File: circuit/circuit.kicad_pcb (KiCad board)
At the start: 4 copper layers, 175.5 x 119.5 mm, 206 parts, among them J201 Barrel_Jack, J301 FX_R_2, J302 FX_R_4, J303 FX_R_6, J304 FX_R_8, J305 FX_R_1, J306 FX_R_3, J307 FX_R_5, J308 FX_R_7, J309 FX_S_1, J310 FX_S_2, J311 FX_S_3, J312 FX_S_4, J313 FX_S_5, J314 FX_S_6, J315 FX_S_7, J316 FX_S_8, J317 Guitar_In, J318 Amp_Out, SW101 Pedal_1, SW102 Pedal_2, SW103 Pedal_3, SW104 Pedal_4, SW105 Pedal_5, SW106 Pedal_6, SW107 Pedal_7, SW108 Pedal_8, SW109 Program, SW110 Preset, U101 ESP32-S3-DevKitC, U201 TMA-1215D, U202 LM7805_TO220, U203 LM7905_TO220, U204 LM1117T-3.3, U301 TL072, U302 TL072, U303 TL072, U304 TL072, U305 TL072, U306 TL072, U307 TL072, U308 TL072, U309 TL072, U401 ADG419BN, U402 CD4051B, U501 CD4051B, U502 CD4051B, U503 CD4051B, U504 CD4051B, U601 CD4051B, U602 CD4051B, U603 CD4051B, U604 CD4051B, U701 74HC595, U702 74HC595, U703 74HC595, U704 74HC595, U801 74HC595, U802 74HC595, U901 74HC595, U902 74HC595

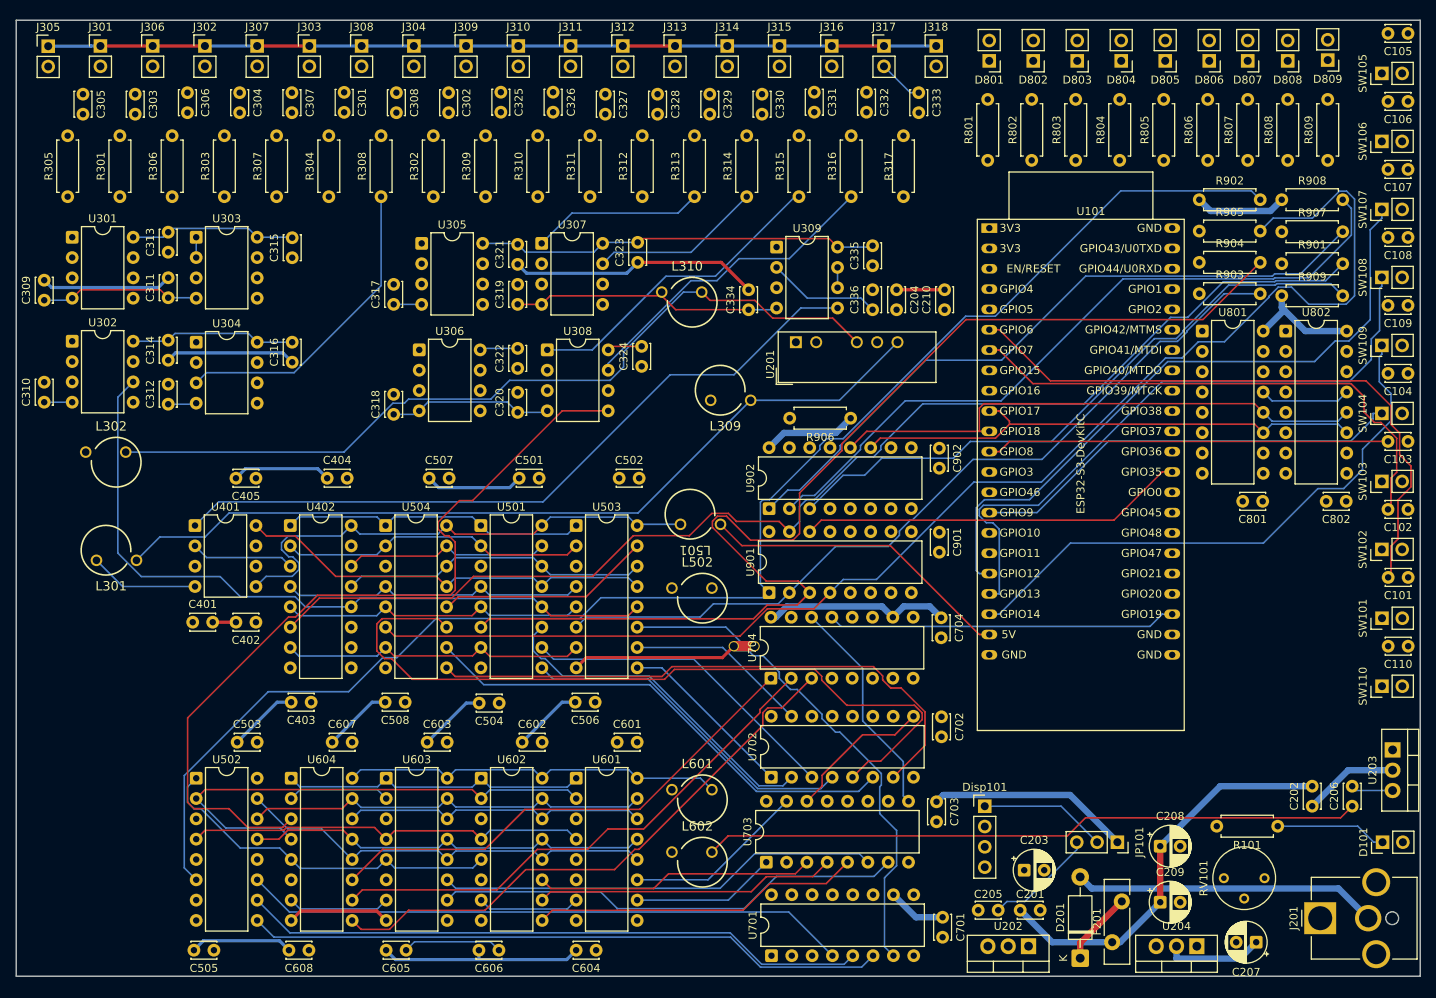
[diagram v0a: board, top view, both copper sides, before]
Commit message: Circuit tweaks and PCB
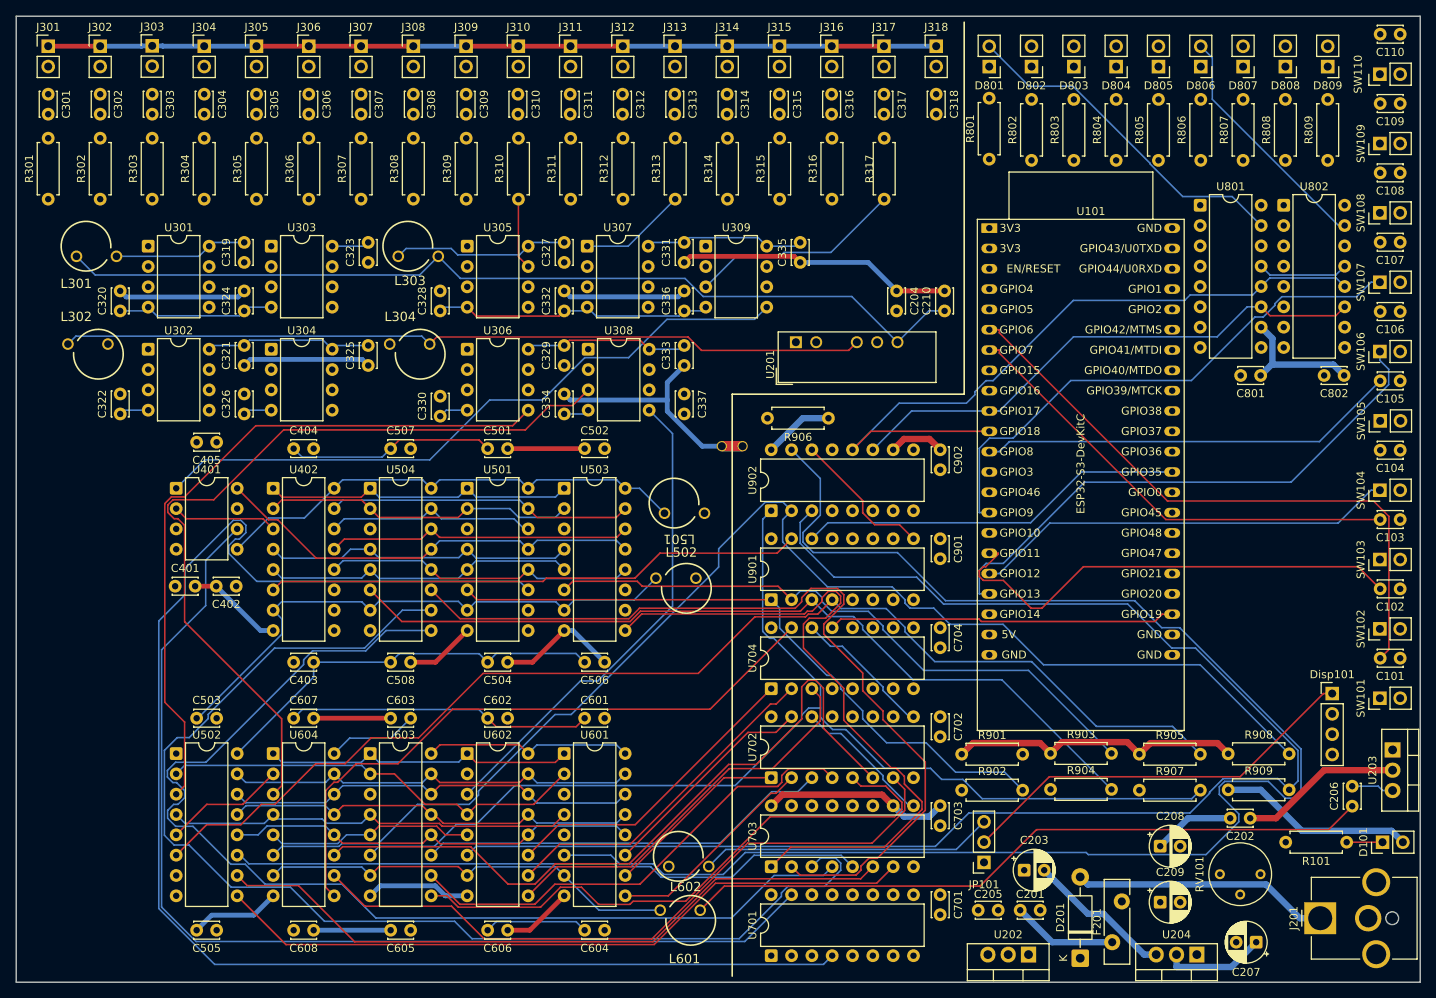
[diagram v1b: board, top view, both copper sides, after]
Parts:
- removed L309, L310: 600R@100Mhz, WE-UKW:WE-UKW_74275010
- added C337: 1uF, Capacitor_THT:C_Disc_D3.0mm_W2.0mm_P2.50mm, F.Cu at (122.0, 84.0)
- added L303: 600R@100Mhz, WE-UKW:WE-UKW_74275010, F.Cu at (87.5, 65.5)
- added L304: 600R@100Mhz, WE-UKW:WE-UKW_74275010, F.Cu at (89.0, 79.0)
- C309, C310, C311, C312, C313, C314, C315, C316, C317, C318: value 0.1uF -> 1uF
- C325, C326, C327, C328, C329, C330, C331, C332, C333, C336: value 1uF -> 0.1uF
- D201: value 1N4007 -> 1N5822
- J301: value FX_R_2 -> FX_R_1
- J302: value FX_R_4 -> FX_R_2
- J303: value FX_R_6 -> FX_R_3
- J304: value FX_R_8 -> FX_R_4
- J305: value FX_R_1 -> FX_R_5
- J306: value FX_R_3 -> FX_R_6
- J307: value FX_R_5 -> FX_R_7
- J308: value FX_R_7 -> FX_R_8
- SW102: value Pedal_2 -> Pedal_6
- SW103: value Pedal_3 -> Pedal_2
- SW104: value Pedal_4 -> Pedal_7
- SW105: value Pedal_5 -> Pedal_3
- SW106: value Pedal_6 -> Pedal_8
- SW107: value Pedal_7 -> Pedal_4
- SW108: value Pedal_8 -> Program
- SW109: value Program -> Pedal_5
- moved R902 79.6 mm to (156.7, 133.5)
- moved C318 78.7 mm to (153.5, 46.5), turned to -90 degrees
- moved C314 77.4 mm to (127.4, 46.5), turned to -90 degrees
- moved C110 76.5 mm to (211.5, 39.0)
- moved SW110 76.5 mm to (209.0, 44.0)
- moved C316 75.3 mm to (140.4, 46.5), turned to -90 degrees
- moved R901 73.2 mm to (156.7, 129.0)
- moved R907 72.0 mm to (178.9, 133.5)
- moved C310 70.6 mm to (101.2, 46.5), turned to -90 degrees
- moved R908 69.6 mm to (190.0, 128.9)
- moved C312 68.7 mm to (114.3, 46.5), turned to -90 degrees
- moved R904 68.4 mm to (167.8, 133.4)
- moved C317 66.7 mm to (147.0, 46.5), turned to -90 degrees
- moved C313 66.3 mm to (120.8, 46.5), turned to -90 degrees
- moved R905 65.8 mm to (178.9, 129.0)
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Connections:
- C102 pad 2: Net-(U101-GPIO7/ADC1_CH6) -> Net-(U101-GPIO11/ADC2_CH0)
- C103 pad 2: Net-(U101-GPIO8/ADC1_CH7) -> Net-(U101-GPIO7/ADC1_CH6)
- C104 pad 2: Net-(U101-GPIO9/ADC1_CH8) -> Net-(U101-GPIO12/ADC2_CH1)
- C105 pad 2: Net-(U101-GPIO10/ADC1_CH9) -> Net-(U101-GPIO8/ADC1_CH7)
- C106 pad 2: Net-(U101-GPIO11/ADC2_CH0) -> Net-(U101-GPIO13/ADC2_CH2)
- C107 pad 2: Net-(U101-GPIO12/ADC2_CH1) -> Net-(U101-GPIO9/ADC1_CH8)
- C108 pad 2: Net-(U101-GPIO13/ADC2_CH2) -> Net-(U101-GPIO14/ADC2_CH3)
- C109 pad 2: Net-(U101-GPIO14/ADC2_CH3) -> Net-(U101-GPIO10/ADC1_CH9)
- C309 pad 1: _15V_F -> Net-(C309-Pad1)
- C309 pad 2: AGND -> Net-(C309-Pad2)
- C310 pad 1: _15V_F -> Net-(C310-Pad1)
- C310 pad 2: AGND -> Net-(C310-Pad2)
- C311 pad 1: _15V_F -> Net-(C311-Pad1)
- C311 pad 2: AGND -> Net-(C311-Pad2)
- C312 pad 1: _15V_F -> Net-(C312-Pad1)
- C312 pad 2: AGND -> Net-(C312-Pad2)
- C313 pad 1: AGND -> Net-(C313-Pad1)
- C313 pad 2: +15V_F -> Net-(C313-Pad2)
- C314 pad 1: AGND -> Net-(C314-Pad1)
- C314 pad 2: +15V_F -> Net-(C314-Pad2)
- C315 pad 1: AGND -> Net-(C315-Pad1)
- C315 pad 2: +15V_F -> Net-(C315-Pad2)
- C316 pad 1: AGND -> Net-(C316-Pad1)
- C316 pad 2: +15V_F -> Net-(C316-Pad2)
- C317 pad 1: Net-(U305-V-) -> Net-(C317-Pad1)
- C317 pad 2: AGND -> Net-(C317-Pad2)
- C318 pad 1: Net-(U305-V-) -> Net-(C318-Pad1)
- C318 pad 2: AGND -> Net-(U309-2-)
- C319 pad 1: Net-(U305-V-) -> AGND
- C319 pad 2: AGND -> +15V_F
- C320 pad 1: Net-(U305-V-) -> -15V_F
- C321 pad 2: Net-(U305-V+) -> +15V_F
- C322 pad 1: AGND -> -15V_F
- C322 pad 2: Net-(U305-V+) -> AGND
- C323 pad 2: Net-(U305-V+) -> +15V_F
- C324 pad 1: AGND -> -15V_F
- C324 pad 2: Net-(U305-V+) -> AGND
- C325 pad 1: Net-(C325-Pad1) -> AGND
- C325 pad 2: Net-(C325-Pad2) -> +15V_F
- C326 pad 1: Net-(C326-Pad1) -> -15V_F
- C326 pad 2: Net-(C326-Pad2) -> AGND
- C327 pad 1: Net-(C327-Pad1) -> AGND
- C327 pad 2: Net-(C327-Pad2) -> Net-(U305-V+)
- C328 pad 1: Net-(C328-Pad1) -> Net-(U305-V-)
- C328 pad 2: Net-(C328-Pad2) -> AGND
- C329 pad 1: Net-(C329-Pad1) -> AGND
- C329 pad 2: Net-(C329-Pad2) -> Net-(U305-V+)
- C330 pad 1: Net-(C330-Pad1) -> Net-(U305-V-)
- C330 pad 2: Net-(C330-Pad2) -> AGND
- C331 pad 1: Net-(C331-Pad1) -> AGND
- C331 pad 2: Net-(C331-Pad2) -> Net-(U305-V+)
- C332 pad 1: Net-(C332-Pad1) -> Net-(U305-V-)
- C332 pad 2: Net-(C332-Pad2) -> AGND
- C333 pad 1: Net-(C333-Pad1) -> AGND
- C333 pad 2: Net-(C333-Pad2) -> Net-(U305-V+)
- C336 pad 1: Net-(U309-1-) -> Net-(U305-V-)
- C336 pad 2: GUITAR_IN -> AGND
- C402 pad 1: +5V_F -> -15V_F
- C403 pad 1: -5V_F -> +5V_F
- C404 pad 1: AGND -> -5V_F
- C404 pad 2: +5V_F -> AGND
- C405 pad 1: -15V_F -> AGND
- C405 pad 2: AGND -> +5V_F
- C501 pad 1: AGND -> -5V_F
- C501 pad 2: +5V_F -> AGND
- C503 pad 1: AGND -> -5V_F
- C503 pad 2: +5V_F -> AGND
- C504 pad 1: -5V_F -> AGND
- C504 pad 2: AGND -> +5V_F
- C506 pad 1: -5V_F -> AGND
- C506 pad 2: AGND -> +5V_F
- C507 pad 1: AGND -> -5V_F
- C507 pad 2: +5V_F -> AGND
- C508 pad 1: -5V_F -> AGND
- C508 pad 2: AGND -> +5V_F
- C601 pad 1: AGND -> Net-(U601-VEE)
- C601 pad 2: Net-(U601-VDD) -> AGND
- C602 pad 1: AGND -> Net-(U601-VEE)
- C602 pad 2: Net-(U601-VDD) -> AGND
- C604 pad 1: Net-(U601-VEE) -> AGND
- C604 pad 2: AGND -> Net-(U601-VDD)
- C606 pad 1: Net-(U601-VEE) -> AGND
- C606 pad 2: AGND -> Net-(U601-VDD)
- C607 pad 1: AGND -> Net-(U601-VEE)
- C607 pad 2: Net-(U601-VDD) -> AGND
- C608 pad 1: Net-(U601-VEE) -> AGND
- C608 pad 2: AGND -> Net-(U601-VDD)
- J201 pad 1: GND -> /Power/12V_RAW_1
- J201 pad 2: /Power/12V_RAW_1 -> GND
- J301 pad T: Net-(C303-Pad1) -> Net-(C301-Pad1)
- J302 pad T: Net-(C304-Pad1) -> Net-(C302-Pad1)
- J303 pad T: Net-(C301-Pad1) -> Net-(C303-Pad1)
- J304 pad T: Net-(C302-Pad1) -> Net-(C304-Pad1)
- J309 pad T: Net-(C325-Pad1) -> Net-(C309-Pad1)
- J310 pad T: Net-(C326-Pad1) -> Net-(C310-Pad1)
- J311 pad T: Net-(C327-Pad1) -> Net-(C311-Pad1)
- J312 pad T: Net-(C328-Pad1) -> Net-(C312-Pad1)
- J313 pad T: Net-(C329-Pad1) -> Net-(C313-Pad1)
- J314 pad T: Net-(C330-Pad1) -> Net-(C314-Pad1)
- J315 pad T: Net-(C331-Pad1) -> Net-(C315-Pad1)
- J316 pad T: Net-(C332-Pad1) -> Net-(C316-Pad1)
- J317 pad T: Net-(C333-Pad1) -> Net-(C317-Pad1)
- J318 pad T: Net-(U309-2-) -> Net-(C318-Pad1)
- L301 pad 1: +15V -> +15V_F
- L301 pad 2: +15V_F -> +15V
- L302 pad 1: _15V_F -> -15V
- L302 pad 2: -15V -> -15V_F
- R301 pad 1: Net-(U301-2+) -> Net-(U301-1+)
- R301 pad 2: Net-(C303-Pad2) -> Net-(C301-Pad2)
- R302 pad 1: Net-(U304-2+) -> Net-(U301-2+)
- R303 pad 1: Net-(U302-2+) -> Net-(U302-1+)
- R303 pad 2: Net-(C304-Pad2) -> Net-(C303-Pad2)
- R304 pad 1: Net-(U303-2+) -> Net-(U302-2+)
- R304 pad 2: Net-(C301-Pad2) -> Net-(C304-Pad2)
- R305 pad 1: Net-(U301-1+) -> Net-(U303-1+)
- R306 pad 1: Net-(U302-1+) -> Net-(U303-2+)
- R307 pad 1: Net-(U303-1+) -> Net-(U304-1+)
- R308 pad 1: Net-(U304-1+) -> Net-(U304-2+)
- R309 pad 2: Net-(C325-Pad2) -> Net-(C309-Pad2)
- R310 pad 2: Net-(C326-Pad2) -> Net-(C310-Pad2)
- R311 pad 2: Net-(C327-Pad2) -> Net-(C311-Pad2)
- R312 pad 2: Net-(C328-Pad2) -> Net-(C312-Pad2)
- R313 pad 2: Net-(C329-Pad2) -> Net-(C313-Pad2)
- R314 pad 2: Net-(C330-Pad2) -> Net-(C314-Pad2)
- R315 pad 2: Net-(C331-Pad2) -> Net-(C315-Pad2)
- R316 pad 2: Net-(C332-Pad2) -> Net-(C316-Pad2)
- R317 pad 2: Net-(C333-Pad2) -> Net-(C317-Pad2)
- SW102 pad 1: Net-(U101-GPIO7/ADC1_CH6) -> Net-(U101-GPIO11/ADC2_CH0)
- SW103 pad 1: Net-(U101-GPIO8/ADC1_CH7) -> Net-(U101-GPIO7/ADC1_CH6)
- SW104 pad 1: Net-(U101-GPIO9/ADC1_CH8) -> Net-(U101-GPIO12/ADC2_CH1)
- SW105 pad 1: Net-(U101-GPIO10/ADC1_CH9) -> Net-(U101-GPIO8/ADC1_CH7)
- SW106 pad 1: Net-(U101-GPIO11/ADC2_CH0) -> Net-(U101-GPIO13/ADC2_CH2)
- SW107 pad 1: Net-(U101-GPIO12/ADC2_CH1) -> Net-(U101-GPIO9/ADC1_CH8)
- SW108 pad 1: Net-(U101-GPIO13/ADC2_CH2) -> Net-(U101-GPIO14/ADC2_CH3)
- SW109 pad 1: Net-(U101-GPIO14/ADC2_CH3) -> Net-(U101-GPIO10/ADC1_CH9)
- U301 pad 4: _15V_F -> -15V_F
- U302 pad 4: _15V_F -> -15V_F
- U303 pad 4: _15V_F -> -15V_F
- U304 pad 4: _15V_F -> -15V_F
- U501 pad 10: /Matrix Shift Registers/U8_Q3 -> /IO Routing/U7_Q5
- U501 pad 11: /Matrix Shift Registers/U8_Q2 -> /IO Routing/U7_Q4
- U501 pad 14: FX_R_1 -> FX_R_2
- U501 pad 15: FX_R_2 -> FX_R_3
- U501 pad 3: FX_S_3 -> FX_S_1
- U501 pad 6: /IO Routing/U901_Q3 -> /IO Routing/U901_Q1
- U501 pad 9: /Matrix Shift Registers/U8_Q4 -> /IO Routing/U7_Q6
- U502 pad 10: /IO Routing/U7_Q5 -> /Matrix Shift Registers/U8_Q6
- U502 pad 11: /IO Routing/U7_Q4 -> /Matrix Shift Registers/U8_Q5
- U502 pad 12: FX_R_4 -> FX_R_3
- U502 pad 14: FX_R_2 -> FX_R_1
- U502 pad 15: FX_R_3 -> FX_R_2
- U502 pad 3: FX_S_1 -> FX_S_4
- U502 pad 6: /IO Routing/U901_Q1 -> /IO Routing/U901_Q4
- U502 pad 9: /IO Routing/U7_Q6 -> /Matrix Shift Registers/U8_Q7
- U504 pad 10: /Matrix Shift Registers/U8_Q6 -> /Matrix Shift Registers/U8_Q3
- U504 pad 11: /Matrix Shift Registers/U8_Q5 -> /Matrix Shift Registers/U8_Q2
- U504 pad 12: FX_R_3 -> FX_R_4
- U504 pad 3: FX_S_4 -> FX_S_3
- U504 pad 6: /IO Routing/U901_Q4 -> /IO Routing/U901_Q3
- U504 pad 9: /Matrix Shift Registers/U8_Q7 -> /Matrix Shift Registers/U8_Q4
- U602 pad 10: /Matrix Shift Registers/U9_Q4 -> /Matrix Shift Registers/U10_Q2
- U602 pad 11: /Matrix Shift Registers/U9_Q3 -> /Matrix Shift Registers/U10_Q1
- U602 pad 2: FX_R_7 -> FX_R_6
- U602 pad 3: FX_S_6 -> FX_S_8
- U602 pad 4: FX_R_8 -> FX_R_7
- U602 pad 6: /Inhibit Registers/U902_Q1 -> /Inhibit Registers/U902_Q3
- U602 pad 9: /Matrix Shift Registers/U9_Q5 -> /Matrix Shift Registers/U10_Q3
- U603 pad 10: /Matrix Shift Registers/U9_Q7 -> /Matrix Shift Registers/U9_Q4
- U603 pad 11: /Matrix Shift Registers/U9_Q6 -> /Matrix Shift Registers/U9_Q3
- U603 pad 2: FX_R_6 -> FX_R_7
- U603 pad 3: FX_S_7 -> FX_S_6
- U603 pad 6: /Inhibit Registers/U902_Q2 -> /Inhibit Registers/U902_Q1
- U603 pad 9: /Matrix Shift Registers/U10_Q0 -> /Matrix Shift Registers/U9_Q5
- U604 pad 10: /Matrix Shift Registers/U10_Q2 -> /Matrix Shift Registers/U9_Q7
- U604 pad 11: /Matrix Shift Registers/U10_Q1 -> /Matrix Shift Registers/U9_Q6
- U604 pad 3: FX_S_8 -> FX_S_7
- U604 pad 4: FX_R_7 -> FX_R_8
- U604 pad 6: /Inhibit Registers/U902_Q3 -> /Inhibit Registers/U902_Q2
- U604 pad 9: /Matrix Shift Registers/U10_Q3 -> /Matrix Shift Registers/U10_Q0
- U702 pad 1: /Matrix Shift Registers/U8_Q1 -> /Matrix Shift Registers/U9_Q1
- U702 pad 14: Net-(U701-QH') -> Net-(U702-SER)
- U702 pad 15: /Matrix Shift Registers/U8_Q0 -> /Matrix Shift Registers/U9_Q0
- U702 pad 2: /Matrix Shift Registers/U8_Q2 -> /Matrix Shift Registers/U9_Q2
- U702 pad 3: /Matrix Shift Registers/U8_Q3 -> /Matrix Shift Registers/U9_Q3
- U702 pad 4: /Matrix Shift Registers/U8_Q4 -> /Matrix Shift Registers/U9_Q4
- U702 pad 5: /Matrix Shift Registers/U8_Q5 -> /Matrix Shift Registers/U9_Q5
- U702 pad 6: /Matrix Shift Registers/U8_Q6 -> /Matrix Shift Registers/U9_Q6
- U702 pad 7: /Matrix Shift Registers/U8_Q7 -> /Matrix Shift Registers/U9_Q7
- U703 pad 1: /Matrix Shift Registers/U9_Q1 -> /Matrix Shift Registers/U8_Q1
- U703 pad 14: Net-(U702-QH') -> Net-(U701-QH')
- U703 pad 15: /Matrix Shift Registers/U9_Q0 -> /Matrix Shift Registers/U8_Q0
- U703 pad 2: /Matrix Shift Registers/U9_Q2 -> /Matrix Shift Registers/U8_Q2
- U703 pad 3: /Matrix Shift Registers/U9_Q3 -> /Matrix Shift Registers/U8_Q3
- U703 pad 4: /Matrix Shift Registers/U9_Q4 -> /Matrix Shift Registers/U8_Q4
- U703 pad 5: /Matrix Shift Registers/U9_Q5 -> /Matrix Shift Registers/U8_Q5
- U703 pad 6: /Matrix Shift Registers/U9_Q6 -> /Matrix Shift Registers/U8_Q6
- U703 pad 7: /Matrix Shift Registers/U9_Q7 -> /Matrix Shift Registers/U8_Q7
- U703 pad 9: Net-(U703-QH') -> Net-(U702-SER)
- U704 pad 14: Net-(U703-QH') -> Net-(U702-QH')
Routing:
- net /Matrix Shift Registers/U8_Q0: track 22.9 -> 162.7 mm
- net /Inhibit Registers/U902_Q0: track 70.7 -> 202.7 mm
- net FX_S_1: track 147.4 -> 31.7 mm
- net /Matrix Shift Registers/U8_Q3: track 40.5 -> 150.4 mm
- net /IO Routing/U7_Q4: track 75.8 -> 185.8 mm
- net /IO Routing/U901_Q1: track 187.3 -> 82.1 mm
- net Net-(Disp101-SDA): track 69.6 -> 168.5 mm
- net /Matrix Shift Registers/U8_Q4: track 43.1 -> 139.8 mm
- net Net-(U101-GPIO14/ADC2_CH3): track 77.2 -> 169.9 mm
- net -15V_F: track 9.39 -> 78.6 mm
- net /Matrix Shift Registers/U8_Q2: track 43.1 -> 109.3 mm
- net /Matrix Shift Registers/U8_Q1: track 22.4 -> 87.6 mm
- net _15V_F: track 62.3 -> 0.00 mm
- net Net-(U101-GPIO15/ADC2_CH4/32K_P): track 147.5 -> 86.1 mm
- net Net-(U601-VDD): track 66.2 -> 127.1 mm
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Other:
- board size 175.5 x 119.5 mm -> 175.5 x 120.8 mm
